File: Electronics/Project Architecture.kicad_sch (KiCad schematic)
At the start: 8 parts

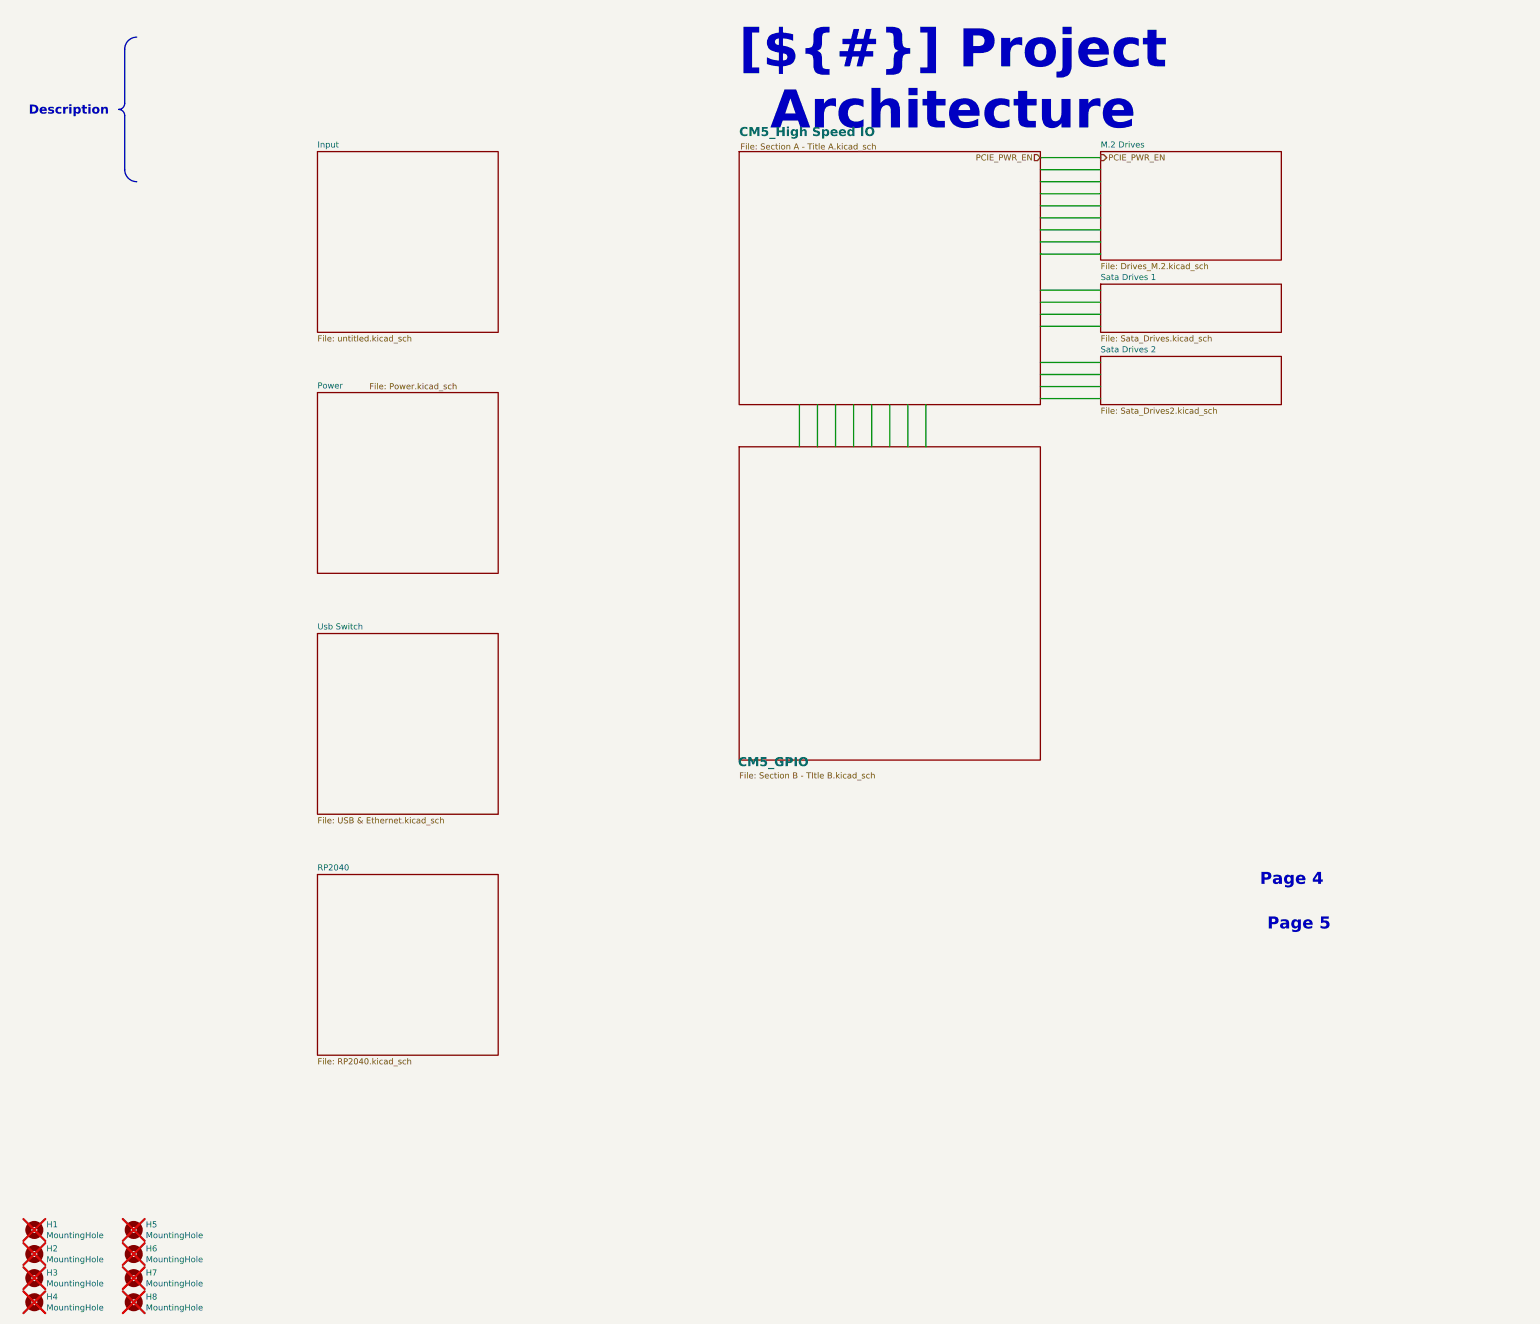
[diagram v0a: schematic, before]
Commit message: Footprints Selected
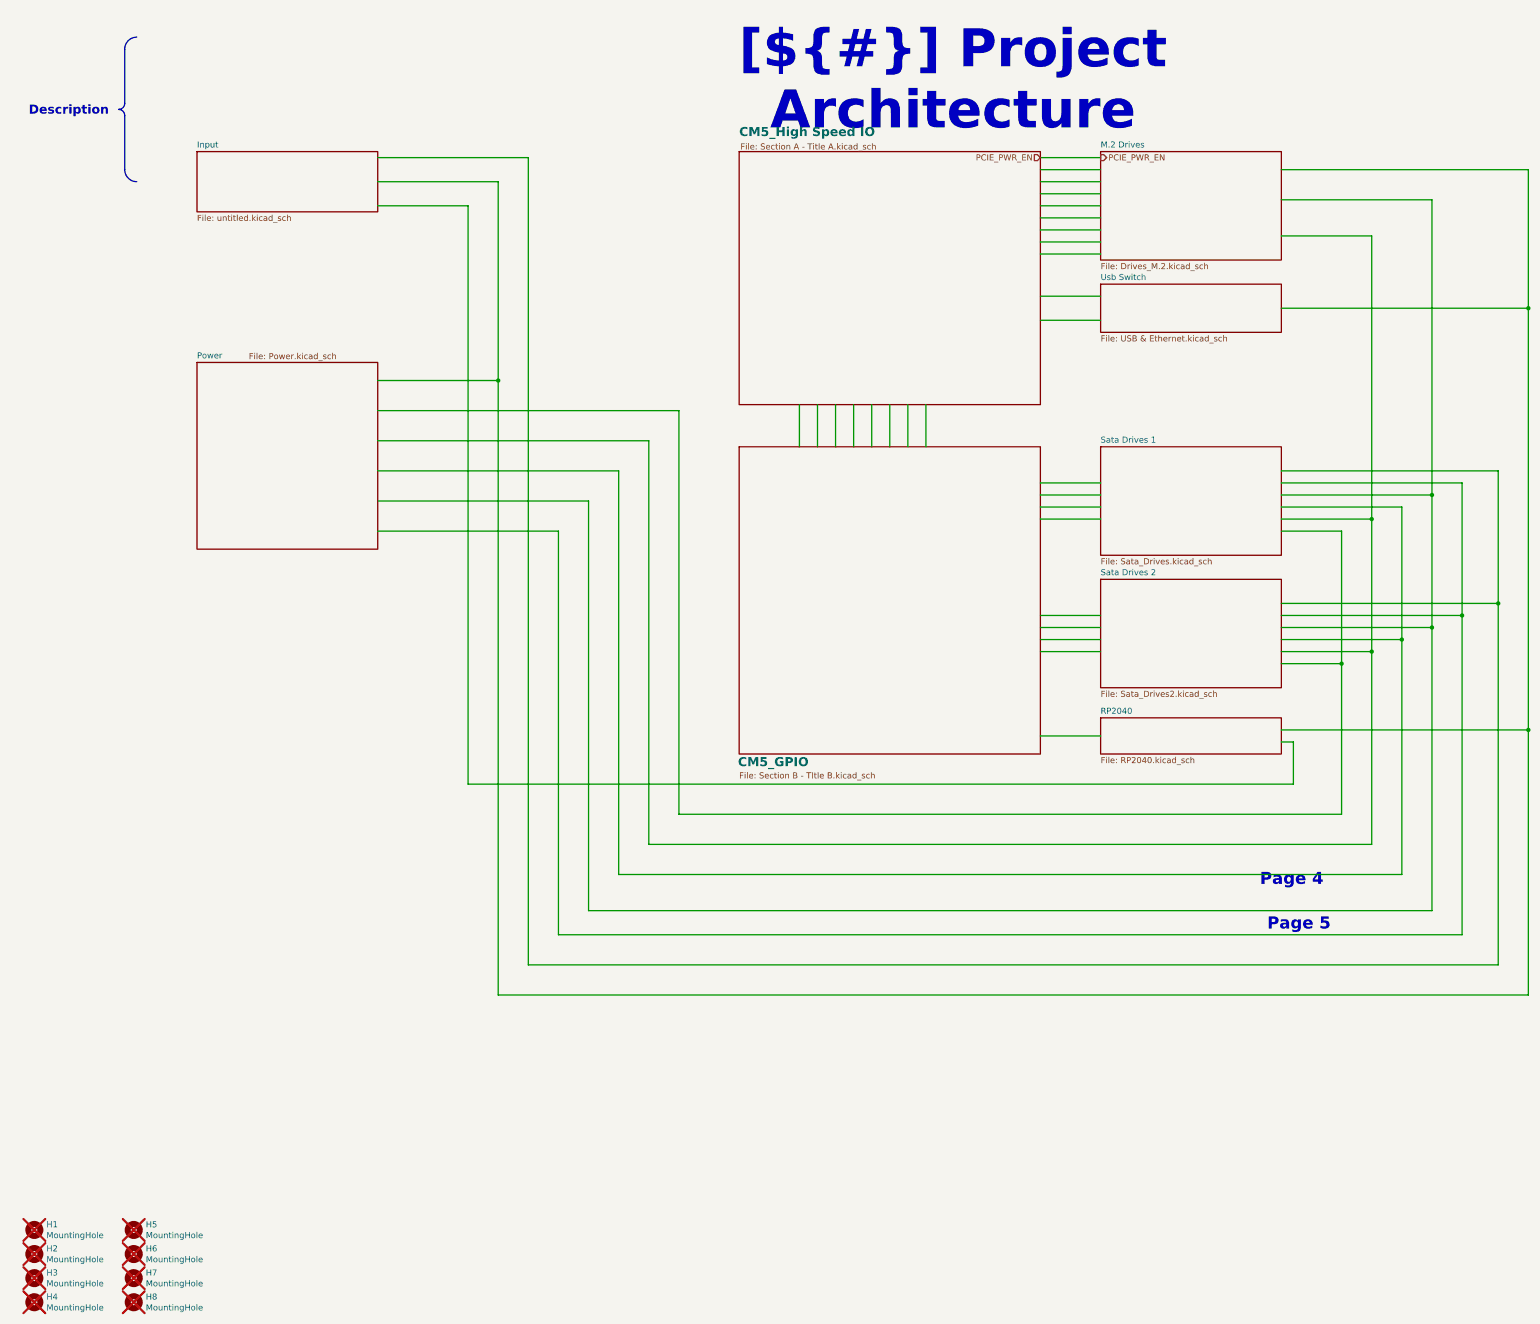
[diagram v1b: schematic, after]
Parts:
- H1, H2, H3, H4, H5, H6, H7, H8: footprint CM5IO:MountingHole_2.7mm_M2.5_DIN965 -> MountingHole:MountingHole_2.7mm_M2.5_DIN965
